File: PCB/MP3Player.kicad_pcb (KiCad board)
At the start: 2 copper layers, 30.5 x 59 mm, 6 parts, among them J1 Raspberry_Pi_4, SW1 RotaryEncoder_Switch, SW2 SW_Push, SW3 SW_Push

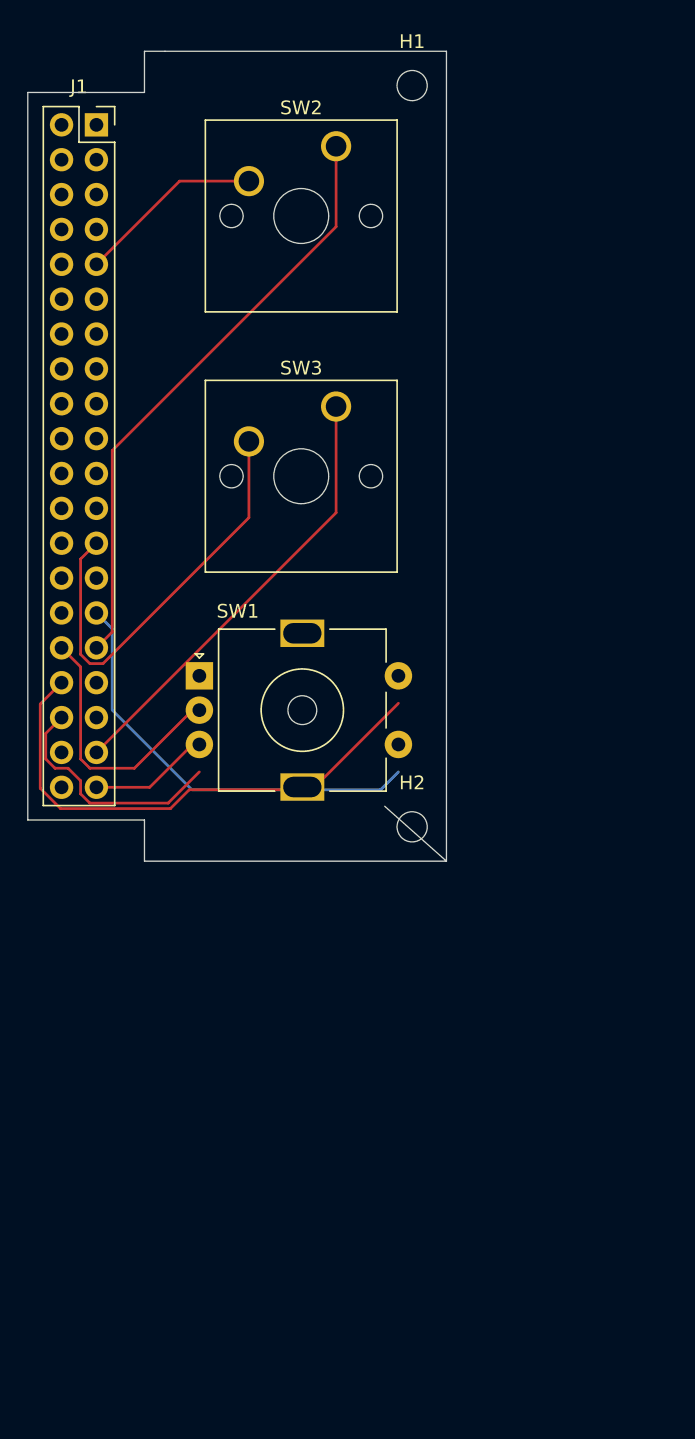
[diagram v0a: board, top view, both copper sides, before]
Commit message: aaaaaa
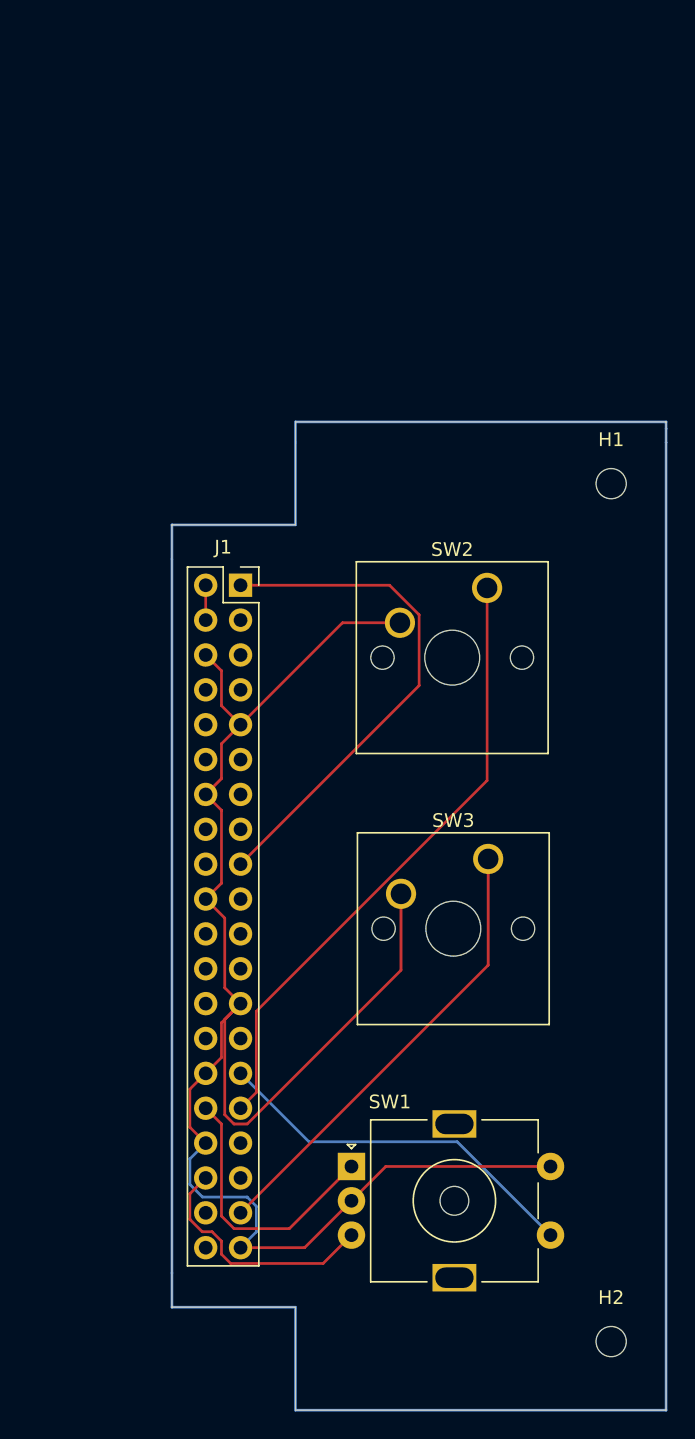
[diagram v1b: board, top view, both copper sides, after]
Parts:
- moved H2 40.2 mm to (170.5, 142.5)
- moved SW1 37.4 mm to (151.6, 129.7)
- moved J1 35.1 mm to (143.5, 87.4)
- moved SW3 34.8 mm to (161.5, 107.3)
- moved SW2 34.0 mm to (161.5, 87.6)
- moved H1 32.4 mm to (170.5, 80.0)
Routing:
- net Net-(J1-3V3-Pad1): track 0.00 -> 37.5 mm
- net Net-(J1-GND-Pad14): track 91.9 -> 125.8 mm
- net Net-(J1-GPCLK1/GPIO05): track 31.3 -> 27.5 mm
- net Net-(J1-5V-Pad2): track 0.00 -> 2.54 mm
- net Net-(J1-GPCLK2/GPIO06): track 43.8 -> 45.3 mm
- net Net-(J1-GPIO26/SDIO_DAT2): track 32.4 -> 33.3 mm
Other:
- board size 30.5 x 59 mm -> 36 x 72 mm
